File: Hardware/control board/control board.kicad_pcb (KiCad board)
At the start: 2 copper layers, 68.1 x 101.7 mm, 37 parts, among them J1 Screw_Terminal_01x02, J10 Screw_Terminal_01x02, J11 Screw_Terminal_01x02, J9 Screw_Terminal_01x02, Q1 NMOS, Q2 NMOS, Q3 NMOS, SW1 SW_Push

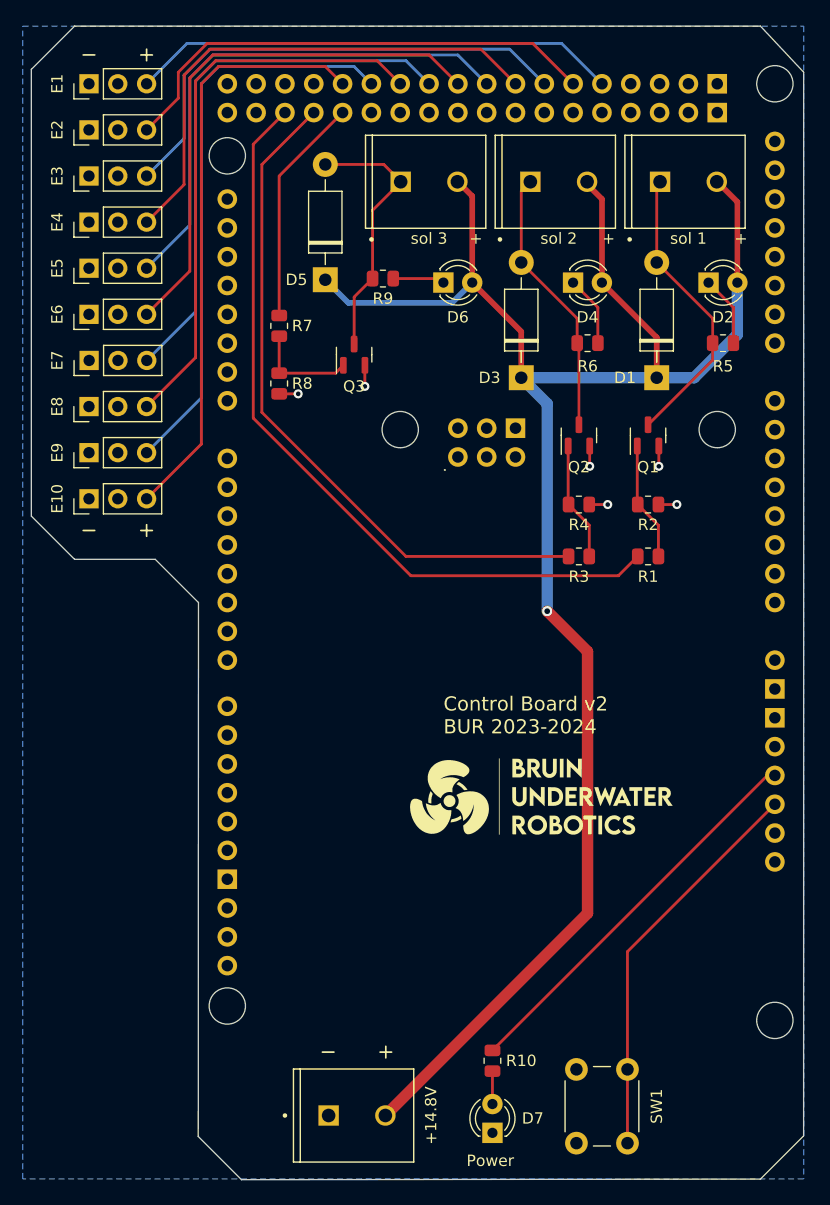
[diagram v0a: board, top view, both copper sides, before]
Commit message: Update control board.kicad_pcb
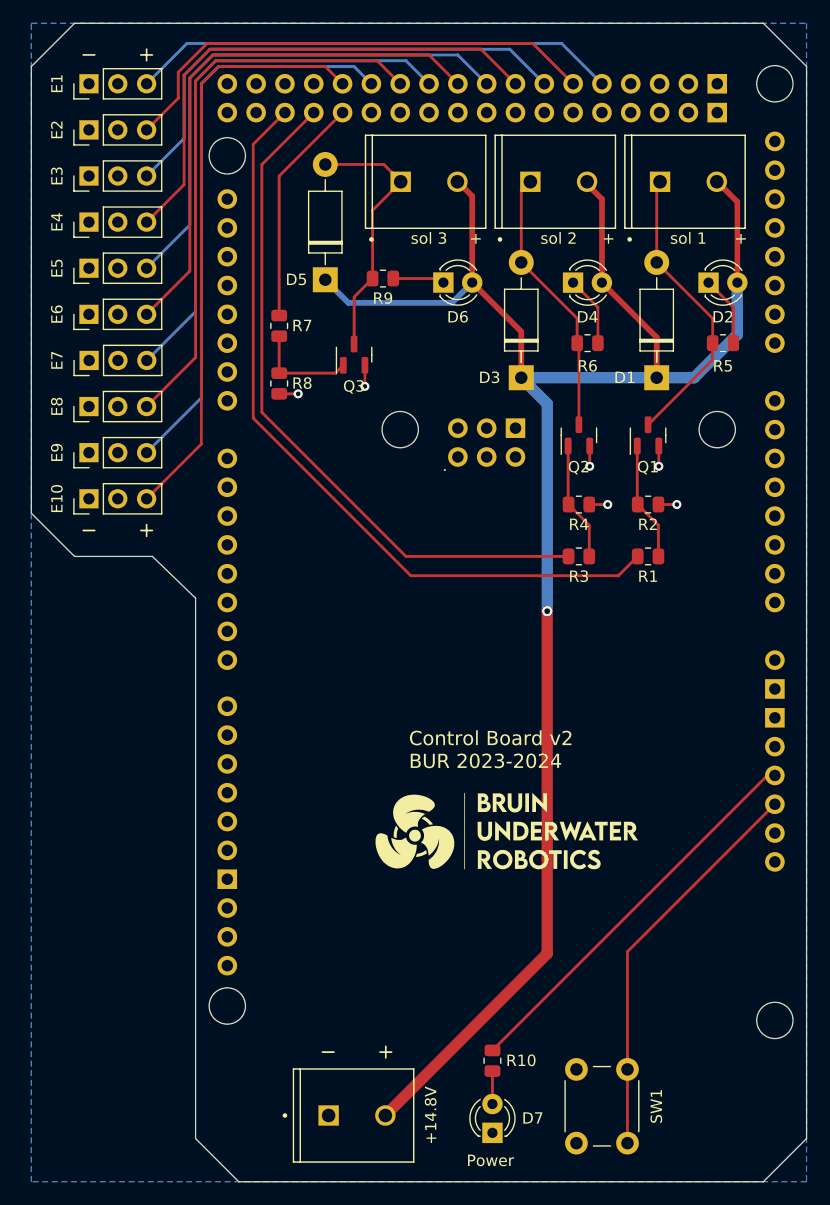
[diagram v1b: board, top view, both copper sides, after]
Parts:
- moved G*** 4.31 mm to (139.7, 111.8)
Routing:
- net +14.8V: track 163.4 -> 160.5 mm
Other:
- board size 68.1 x 101.7 mm -> 68.3 x 102.1 mm
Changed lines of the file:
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@@
   )
   (footprint "LOGO" (layer "F.Cu")
-    (at 142.748 108.712)
+    (at 139.7 111.76)
     (attr board_only exclude_from_pos_files exclude_from_bom)
     (fp_text reference "G***" (at 1.524 -17.272) (layer "F.SilkS") hide
@@
   (gr_line (start 103.378 43.18) (end 102.362 43.18)
     (stroke (width 0.15) (type default)) (layer "F.SilkS"))
-  (gr_line (start 97.79 44.45) (end 97.79 83.82)
+  (gr_line (start 97.79 44.196) (end 97.79 83.566)
     (stroke (width 0.1) (type default)) (layer "Edge.Cuts"))
-  (gr_line (start 97.79 83.82) (end 101.6 87.63)
+  (gr_line (start 97.79 83.566) (end 101.6 87.376)
     (stroke (width 0.1) (type default)) (layer "Edge.Cuts"))
-  (gr_line (start 165.855 138.445) (end 165.862 44.704)
+  (gr_line (start 166.116 138.684) (end 166.116 44.196)
     (stroke (width 0.1) (type default)) (layer "Edge.Cuts"))
-  (gr_line (start 101.6 40.64) (end 111.252 40.64)
+  (gr_line (start 101.6 40.386) (end 111.252 40.386)
     (stroke (width 0.1) (type default)) (layer "Edge.Cuts"))
-  (gr_line (start 165.862 44.704) (end 162.052 40.64)
+  (gr_line (start 166.116 44.196) (end 162.306 40.386)
     (stroke (width 0.1) (type default)) (layer "Edge.Cuts"))
-  (gr_line (start 162.052 40.64) (end 111.252 40.64)
+  (gr_line (start 162.306 40.386) (end 111.252 40.386)
     (stroke (width 0.1) (type default)) (layer "Edge.Cuts"))
-  (gr_line (start 162.045 142.255) (end 165.855 138.445)
+  (gr_line (start 162.306 142.494) (end 166.116 138.684)
     (stroke (width 0.1) (type default)) (layer "Edge.Cuts"))
-  (gr_line (start 112.5 138.5) (end 116.31 142.31)
+  (gr_line (start 112.268 138.684) (end 116.078 142.494)
     (stroke (width 0.1) (type default)) (layer "Edge.Cuts"))
-  (gr_line (start 101.6 40.64) (end 97.79 44.45)
+  (gr_line (start 101.6 40.386) (end 97.79 44.196)
     (stroke (width 0.1) (type default)) (layer "Edge.Cuts"))
-  (gr_line (start 116.31 142.31) (end 162.045 142.255)
+  (gr_line (start 116.078 142.494) (end 162.306 142.494)
     (stroke (width 0.1) (type default)) (layer "Edge.Cuts"))
-  (gr_line (start 108.712 87.63) (end 112.522 91.44)
+  (gr_line (start 108.458 87.376) (end 112.268 91.059)
     (stroke (width 0.1) (type default)) (layer "Edge.Cuts"))
-  (gr_line (start 112.522 91.44) (end 112.5 138.5)
+  (gr_line (start 112.268 91.059) (end 112.268 138.684)
     (stroke (width 0.1) (type default)) (layer "Edge.Cuts"))
-  (gr_line (start 101.6 87.63) (end 108.712 87.63)
+  (gr_line (start 101.6 87.376) (end 108.458 87.376)
     (stroke (width 0.1) (type default)) (layer "Edge.Cuts"))
   (gr_text "+" (at 148.082 59.944) (layer "F.SilkS")
     (effects (font (size 1 1) (thickness 0.15)) (justify left bottom))
   )
-  (gr_text "Control Board v2 \nBUR 2023-2024" (at 134.112 103.124) (layer "F.SilkS")
+  (gr_text "Control Board v2 \nBUR 2023-2024" (at 131.064 106.172) (layer "F.SilkS")
     (effects (font (size 1.25 1.25) (thickness 0.2)) (justify left bottom))
   )
@@
   (segment (start 160.015 62.992) (end 160.015 56.129) (width 0.5) (layer "F.Cu") (net 52))
   (segment (start 136.647 63.241) (end 140.97 67.564) (width 0.5) (layer "F.Cu") (net 52))
+  (segment (start 143.256 92.202) (end 143.256 122.388) (width 1) (layer "F.Cu") (net 52))
   (segment (start 148.082 63.251) (end 152.908 68.077) (width 0.5) (layer "F.Cu") (net 52))
   (segment (start 152.908 68.077) (end 152.908 71.628) (width 0.5) (layer "F.Cu") (net 52))
@@
   (segment (start 148.082 55.88) (end 148.082 63.251) (width 0.5) (layer "F.Cu") (net 52))
   (segment (start 160.015 56.129) (end 158.242 54.356) (width 0.5) (layer "F.Cu") (net 52))
-  (segment (start 146.812 118.832) (end 128.992 136.652) (width 1) (layer "F.Cu") (net 52))
   (segment (start 136.647 55.621) (end 135.382 54.356) (width 0.5) (layer "F.Cu") (net 52))
   (segment (start 140.97 67.564) (end 140.97 71.628) (width 0.5) (layer "F.Cu") (net 52))
-  (segment (start 143.256 92.202) (end 146.812 95.758) (width 1) (layer "F.Cu") (net 52))
-  (segment (start 146.812 95.758) (end 146.812 118.832) (width 1) (layer "F.Cu") (net 52))
+  (segment (start 143.256 122.388) (end 128.992 136.652) (width 1) (layer "F.Cu") (net 52))
   (segment (start 136.647 63.241) (end 136.647 55.621) (width 0.5) (layer "F.Cu") (net 52))
   (via (at 143.256 92.202) (size 0.9) (drill 0.5) (layers "F.Cu" "B.Cu") (net 52))
@@
     (polygon
       (pts
-        (xy 97.028 40.64)
-        (xy 165.862 40.64)
-        (xy 165.862 142.24)
-        (xy 97.028 142.24)
+        (xy 97.79 40.386)
+        (xy 166.116 40.386)
+        (xy 166.116 142.494)
+        (xy 97.79 142.494)
       )
     )
